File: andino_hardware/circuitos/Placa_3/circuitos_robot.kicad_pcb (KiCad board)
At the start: 2 copper layers, 100 x 80 mm, 20 parts, among them J8 Jack-DC

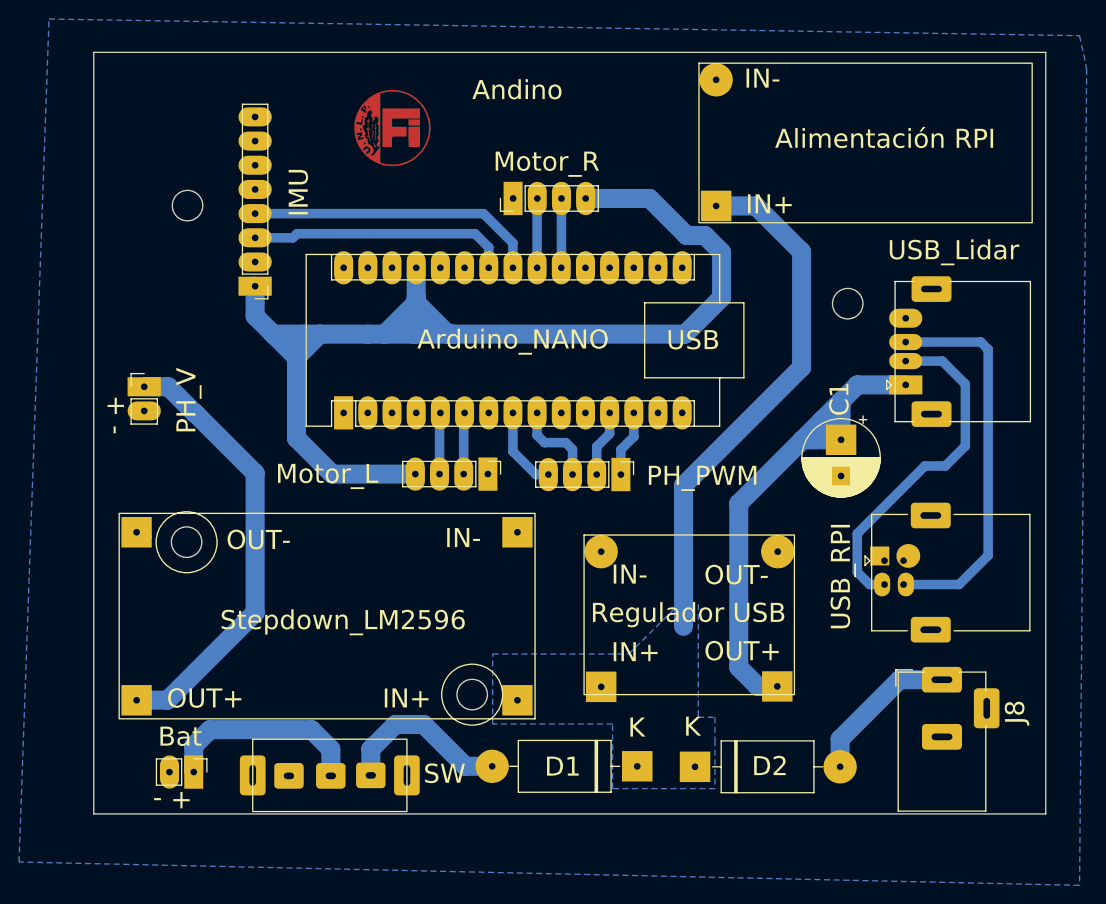
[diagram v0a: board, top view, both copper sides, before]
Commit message: placa
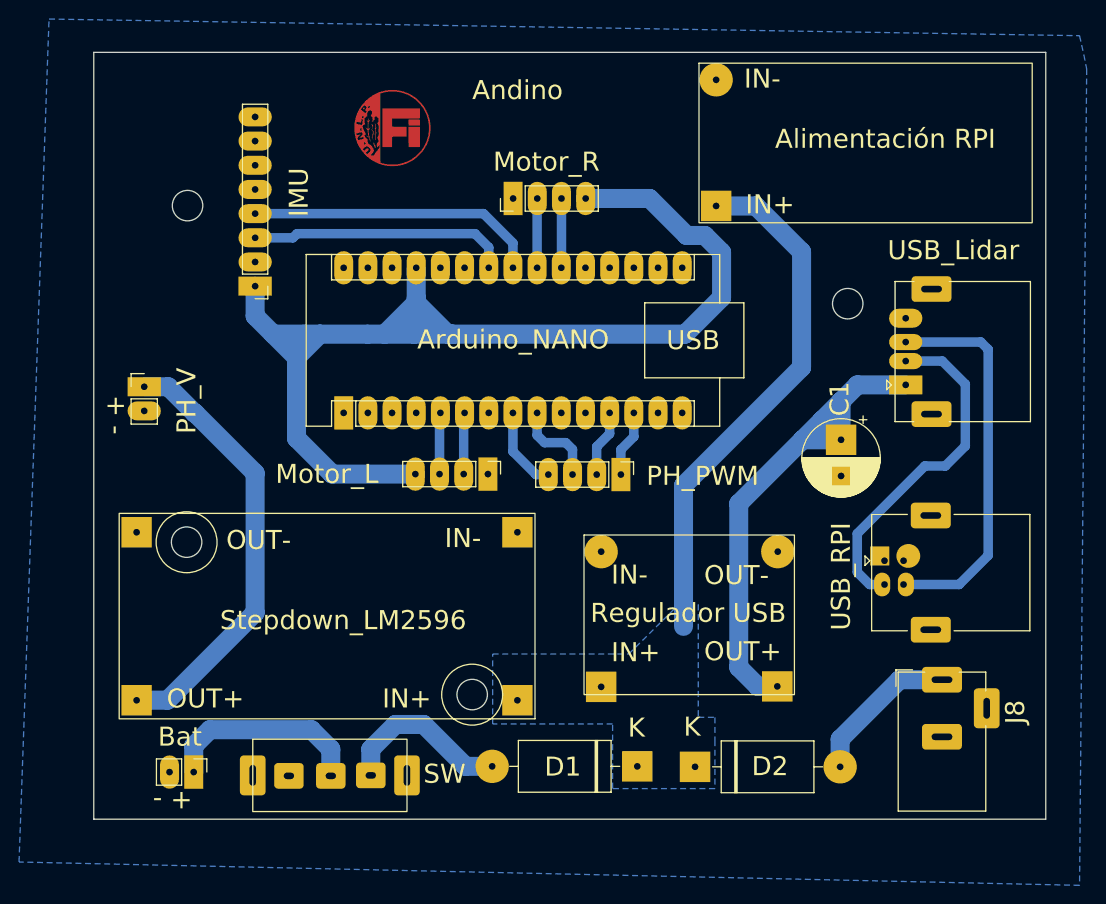
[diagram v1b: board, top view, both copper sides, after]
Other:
- board size 100 x 80 mm -> 100 x 80.5 mm
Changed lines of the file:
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@@
 	(gr_rect
 		(start 24 20.45)
-		(end 124 100.45)
+		(end 124 101)
 		(stroke
 			(width 0.1)
-			(type default)
+			(type solid)
 		)
 		(fill no)
